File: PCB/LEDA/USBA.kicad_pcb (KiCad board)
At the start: 2 copper layers, 70 x 70 mm, 23 parts, among them J1 USB_A, J2 Conn_01x03, U1 ICS43434_MEMS_Mic, U2 ESP32-S3-MINI-1, U5 MD8942

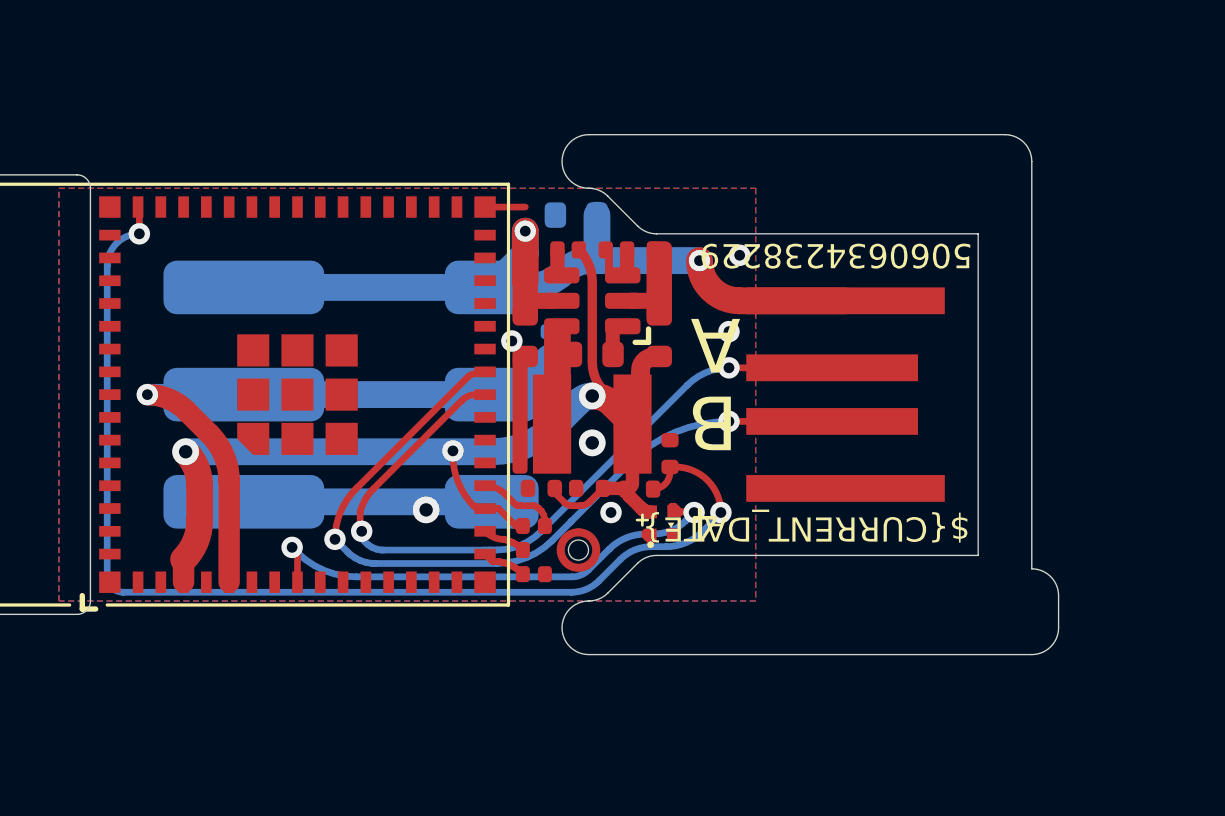
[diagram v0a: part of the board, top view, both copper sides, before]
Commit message: ADC and tidy SS
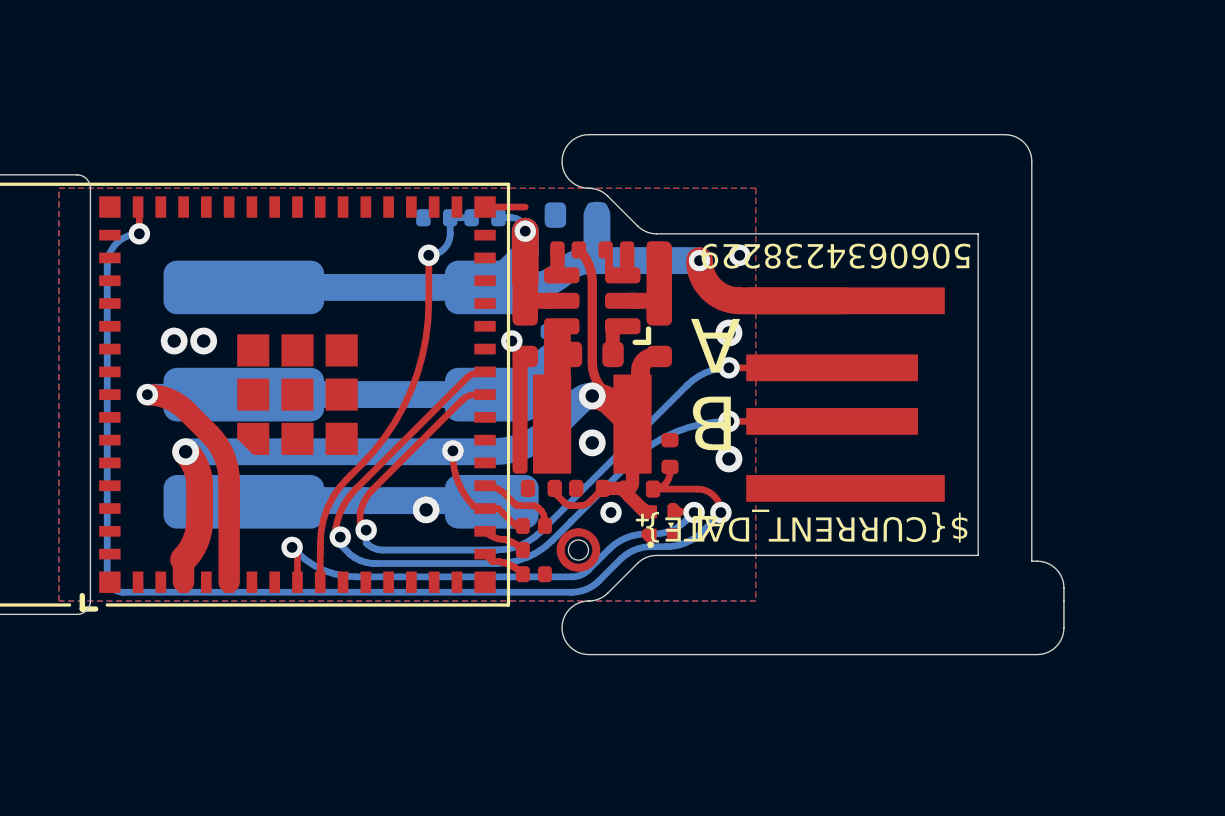
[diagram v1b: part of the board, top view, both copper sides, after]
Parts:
- added R2: 124K, RevK:R_0402, B.Cu at (102.6, 92.7)
- added R3: 10K, RevK:R_0402, B.Cu at (100.8, 92.7)
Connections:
- net VBUS renamed DC
- U2 pad 9: unconnected-(U2-GPIO5-Pad9) -> ADC
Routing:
- net ADC: track 0.00 -> 15.9 mm, vias 0 -> 1
- net DC: track 28.5 -> 29.7 mm
- net GND: vias 6 -> 9
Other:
- board text added: "5"

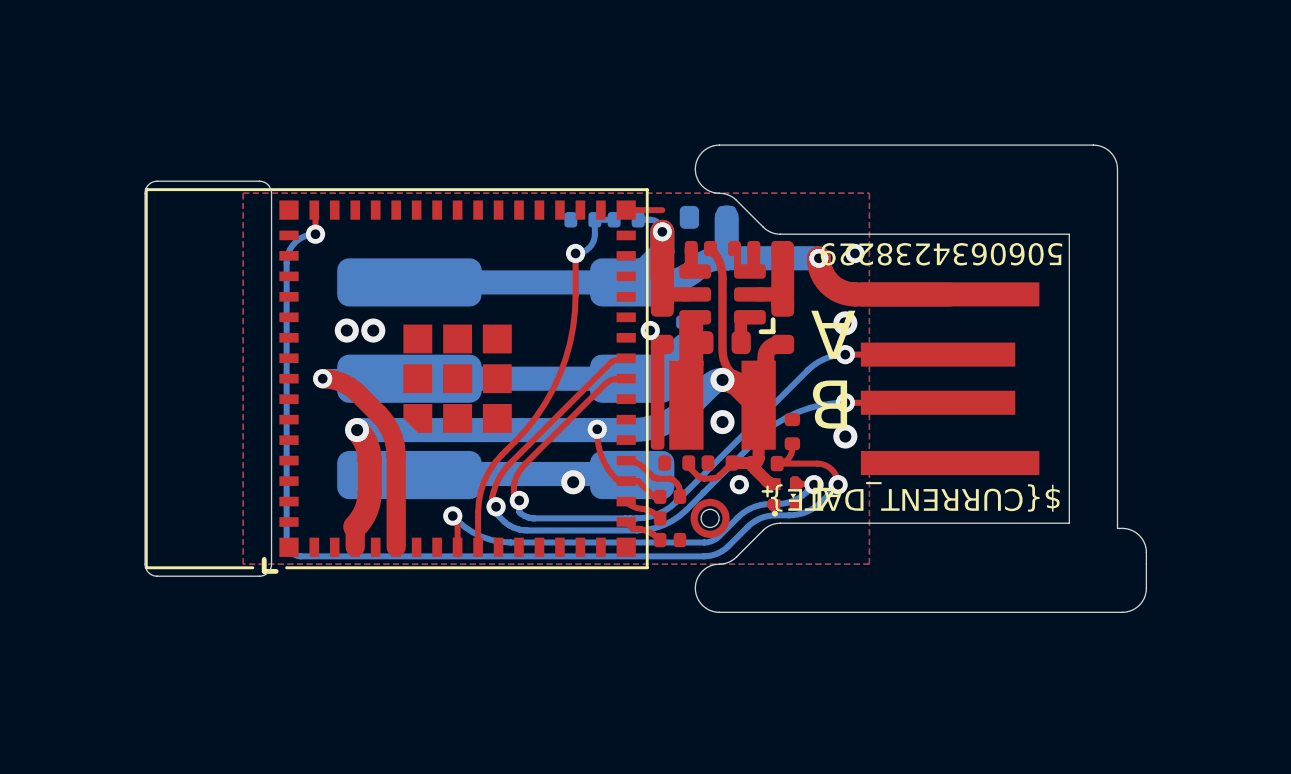
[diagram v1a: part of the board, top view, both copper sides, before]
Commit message: Rework
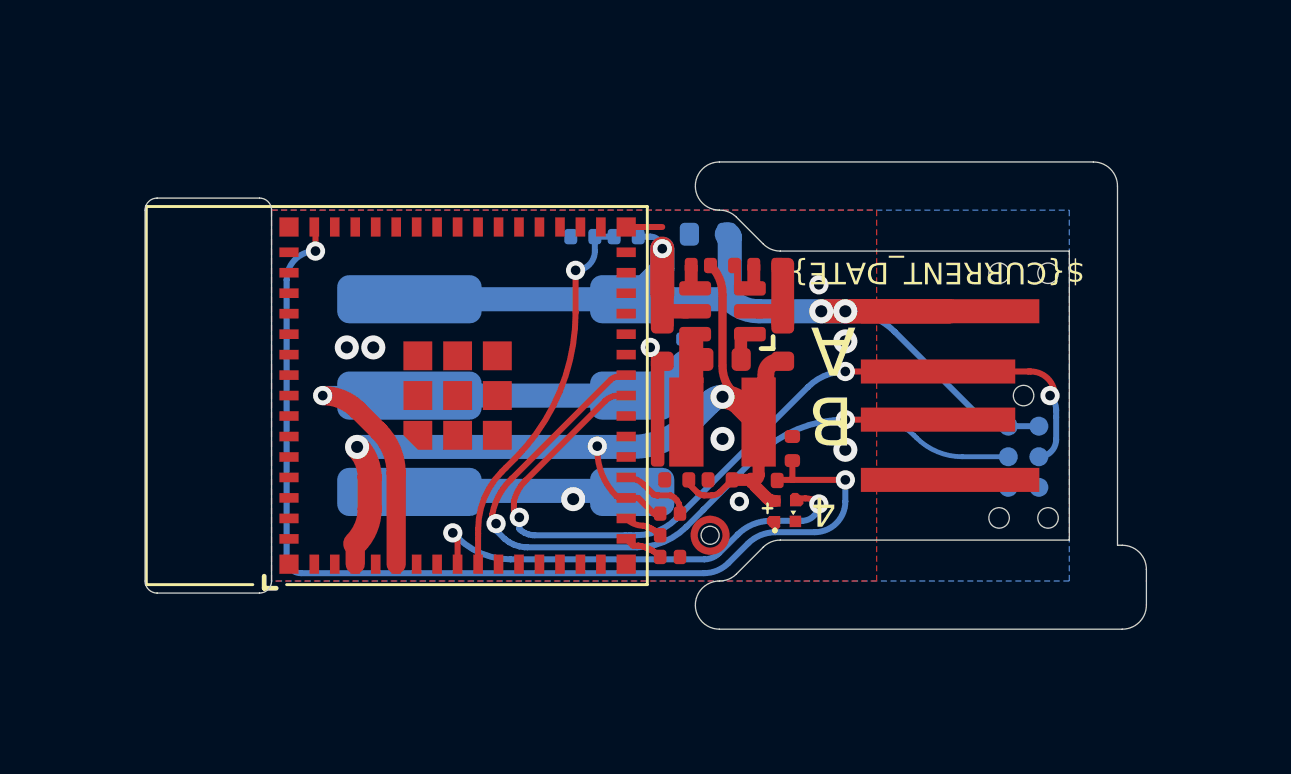
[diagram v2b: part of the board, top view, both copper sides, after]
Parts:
- added ?: , , F.Cu at (119.4, 94.9)
- added ?: , , F.Cu at (116.3, 94.3)
- added J3: TC2030-USB-NL-DS, RevK:Tag-Connect_TC2030-IDC-NL_2x03_P1.27mm_Vertical, B.Cu at (119.1, 102.5)
- moved C1 0.70 mm to (106.5, 103.5)
- moved C2 0.70 mm to (104.7, 103.5)
- moved C3 0.70 mm to (109.5, 102.2)
- moved C4 0.70 mm to (106.0, 93.3)
- moved C6 0.70 mm to (104.1, 97.8)
- moved C7 0.70 mm to (109.1, 97.8)
- moved C8 0.70 mm to (106.6, 98.5)
- moved D1 0.70 mm to (109.2, 104.8)
- moved D2 0.70 mm to (105.0, 98.1)
- moved J1 0.70 mm to (121.0, 100.0)
- moved J2 0.70 mm to (98.2, 100.0)
- moved R1 0.70 mm to (108.4, 103.5)
- moved R2 0.70 mm to (102.6, 93.4)
- moved R3 0.70 mm to (100.8, 93.4)
- moved REF** 0.70 mm to (95.6, 100.0)
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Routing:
- net DC: track 29.7 -> 46.2 mm, vias 2 -> 3
- net D-: track 27.9 -> 36.3 mm, vias 2 -> 3
- net D+: track 29.2 -> 36.3 mm
- net Net-(U2-EN): track 42.7 -> 43.8 mm
- net LED1: track 18.1 -> 18.8 mm
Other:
- board text added: "-HERE-"
- board text added: "Glue tab"
- board text removed: "5060634238229"
- board text removed: "[Glue tab here]"

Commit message: Tryign to do extra holes
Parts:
- removed the ? at (119.4, 94.9)
- removed the ? at (116.3, 94.3)
- added ?: , clipboard:8abff937-711c-455e-bc8a-c75c5e04b52f, F.Cu at (120.1, 94.9)
